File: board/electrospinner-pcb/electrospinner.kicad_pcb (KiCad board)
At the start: 2 copper layers, 50.8 x 38.1 mm, 27 parts, among them J1 Header_02x02, SW1 ResetBTN, U1 FT230XS, U5 MSP430G2553IPW20

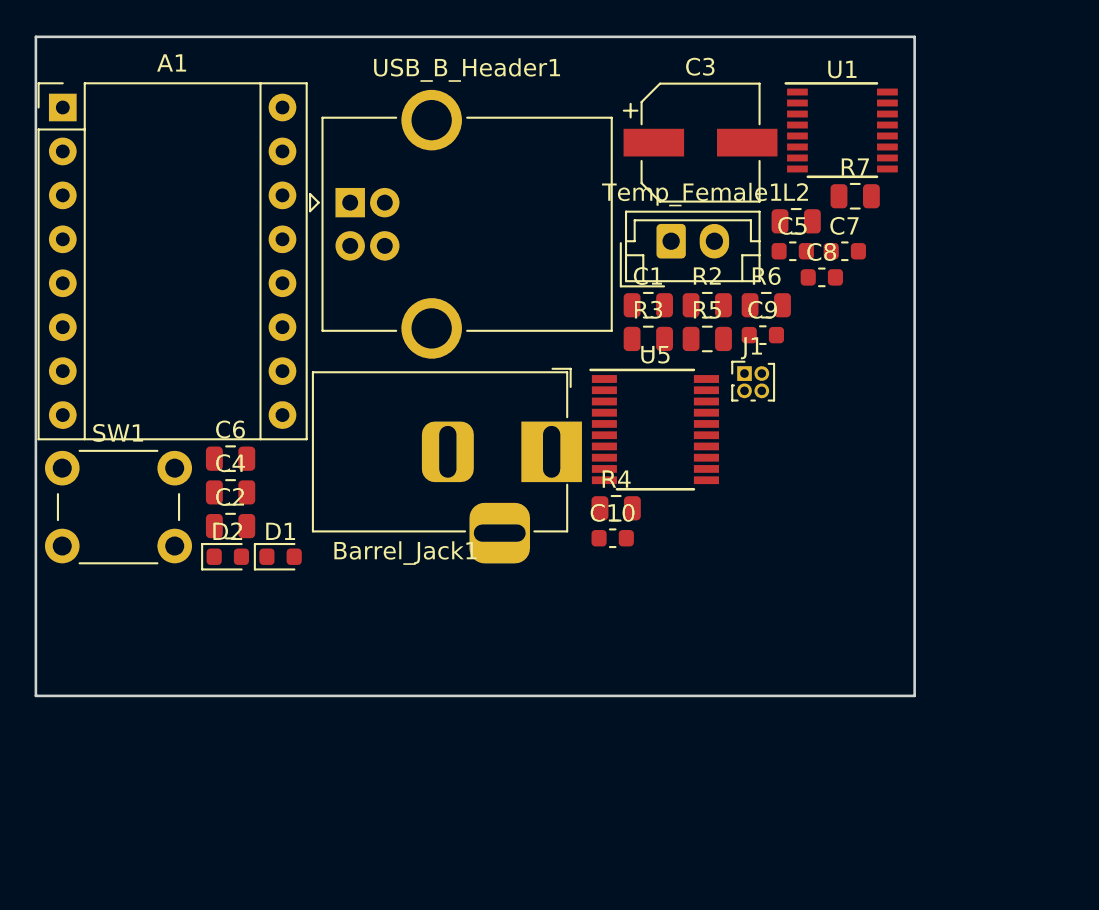
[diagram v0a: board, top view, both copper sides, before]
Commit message: Add files via upload
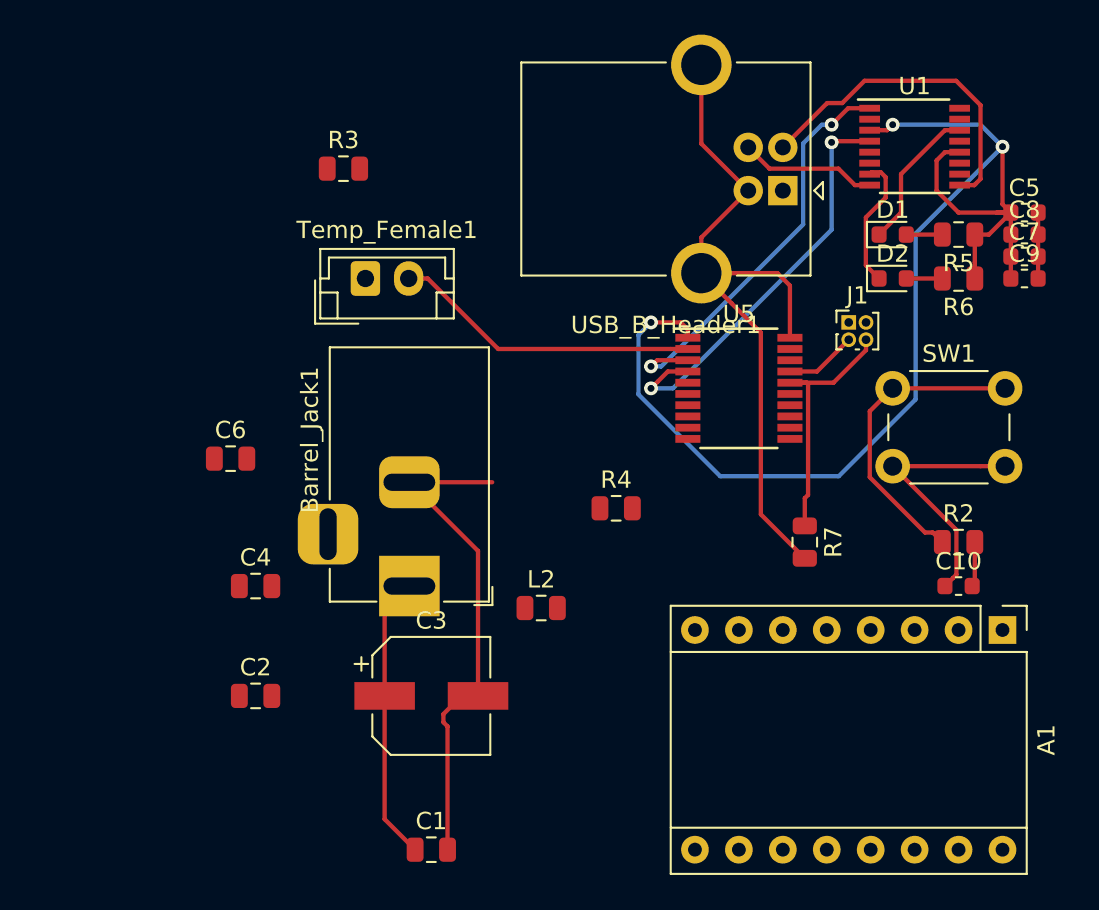
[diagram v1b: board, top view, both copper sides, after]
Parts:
- moved A1 62.2 mm to (182.9, 123.2), turned to 270 degrees
- moved SW1 48.2 mm to (176.5, 109.2)
- moved D2 41.7 mm to (176.5, 102.9)
- moved D1 40.0 mm to (176.5, 100.3)
- moved C3 35.6 mm to (149.9, 127.0)
- moved C1 33.9 mm to (149.9, 135.9)
- moved L2 26.8 mm to (156.2, 121.9)
- moved USB_B_Header1 25.0 mm to (170.2, 97.8), turned to 180 degrees
- moved R7 20.2 mm to (171.4, 118.1), turned to 270 degrees
- moved R3 20.2 mm to (144.8, 96.5)
- moved C10 20.2 mm to (180.3, 120.7)
- moved R2 20.0 mm to (180.3, 118.1)
- moved Temp_Female1 17.8 mm to (146.1, 102.9)
- moved R5 15.7 mm to (180.3, 100.3), turned to 180 degrees
- moved C9 15.5 mm to (184.2, 102.9)
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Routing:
- net +3V3: track 0.00 -> 88.7 mm, vias 0 -> 3
- net GNDD: track 0.00 -> 74.9 mm
- net /~RST: track 0.00 -> 33.1 mm
- net /PCB_RX: track 0.00 -> 24.1 mm, vias 0 -> 2
- net /PCB_TX: track 0.00 -> 23.8 mm, vias 0 -> 2
- net /D-: track 0.00 -> 19.7 mm
- net /Vo,temp: track 0.00 -> 17.8 mm
- net +12V: track 0.00 -> 16.6 mm
- net /~RXLED: track 0.00 -> 8.46 mm
- net /D+: track 0.00 -> 7.92 mm
- net /~TXLED: track 0.00 -> 7.74 mm
- net /TEST: track 0.00 -> 4.16 mm
- net Net-(C10-Pad2): track 0.00 -> 2.60 mm
- net Net-(D2-Pad2): track 0.00 -> 2.09 mm
- net Net-(D1-Pad2): track 0.00 -> 2.09 mm
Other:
- board outline removed
